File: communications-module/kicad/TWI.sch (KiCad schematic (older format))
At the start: 12 parts, among them U10 LIS3DH_breakout, U6 TPS2064, U7 I2C_connector, U8 BME280, U9 I2C_connector

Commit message: Communications Module update
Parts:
- JP17: footprint (none) -> Socket_Strips:Socket_Strip_Straight_1x02_Pitch2.54mm
- U10: footprint LIS3DH_breakout:LIS3DH_breakout -> LIS3DH_breakout:LIS3DH_breakout_vertical
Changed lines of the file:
@@
 $EndComp
 $Comp
-L GND #PWR041
+L GND #PWR50
 U 1 1 589C0F97
 P 4660 2785
-F 0 "#PWR041" H 4660 2535 50  0001 C CNN
+F 0 "#PWR50" H 4660 2535 50  0001 C CNN
 F 1 "GND" H 4660 2635 50  0000 C CNN
 F 2 "" H 4660 2785 60  0000 C CNN
@@
 $EndComp
 $Comp
-L GND #PWR042
+L GND #PWR51
 U 1 1 589C0F9D
 P 5765 2485
-F 0 "#PWR042" H 5765 2235 50  0001 C CNN
+F 0 "#PWR51" H 5765 2235 50  0001 C CNN
 F 1 "GND" H 5765 2335 50  0000 C CNN
 F 2 "" H 5765 2485 60  0000 C CNN
@@
 $EndComp
 $Comp
-L GND #PWR043
+L GND #PWR48
 U 1 1 589C0FAC
 P 4360 2270
-F 0 "#PWR043" H 4360 2020 50  0001 C CNN
+F 0 "#PWR48" H 4360 2020 50  0001 C CNN
 F 1 "GND" H 4360 2120 50  0000 C CNN
 F 2 "" H 4360 2270 60  0000 C CNN
@@
 $EndComp
 $Comp
-L GND #PWR044
+L GND #PWR49
 U 1 1 589C0FC2
 P 4525 3880
-F 0 "#PWR044" H 4525 3630 50  0001 C CNN
+F 0 "#PWR49" H 4525 3630 50  0001 C CNN
 F 1 "GND" H 4525 3730 50  0000 C CNN
 F 2 "" H 4525 3880 60  0000 C CNN
@@
 TWI_SCL
 $Comp
-L GND #PWR045
+L GND #PWR52
 U 1 1 589C0FCA
 P 5970 3885
-F 0 "#PWR045" H 5970 3635 50  0001 C CNN
+F 0 "#PWR52" H 5970 3635 50  0001 C CNN
 F 1 "GND" H 5970 3735 50  0000 C CNN
 F 2 "" H 5970 3885 60  0000 C CNN
@@
 F 0 "U10" H 7660 4860 60  0000 C CNN
 F 1 "LIS3DH_breakout" V 7535 4210 60  0000 C CNN
-F 2 "LIS3DH_breakout:LIS3DH_breakout" V 7435 4210 60  0001 C CNN
+F 2 "LIS3DH_breakout:LIS3DH_breakout_vertical" V 7435 4210 60  0001 C CNN
 F 3 "" H 7810 4710 60  0000 C CNN
 	1    7785 4285
@@
 NoConn ~ 8110 4635
 $Comp
-L GND #PWR046
+L GND #PWR58
 U 1 1 589C0FDB
 P 8580 3935
-F 0 "#PWR046" H 8580 3685 50  0001 C CNN
+F 0 "#PWR58" H 8580 3685 50  0001 C CNN
 F 1 "GND" H 8580 3785 50  0000 C CNN
 F 2 "" H 8580 3935 60  0000 C CNN
@@
 $EndComp
 $Comp
-L GND #PWR047
+L GND #PWR61
 U 1 1 589C0FF3
 P 8870 4595
-F 0 "#PWR047" H 8870 4345 50  0001 C CNN
+F 0 "#PWR61" H 8870 4345 50  0001 C CNN
 F 1 "GND" H 8870 4445 50  0000 C CNN
 F 2 "" H 8870 4595 60  0000 C CNN
@@
 $EndComp
 $Comp
-L GND #PWR048
+L GND #PWR55
 U 1 1 589C1001
 P 7795 3355
-F 0 "#PWR048" H 7795 3105 50  0001 C CNN
+F 0 "#PWR55" H 7795 3105 50  0001 C CNN
 F 1 "GND" H 7795 3205 50  0000 C CNN
 F 2 "" H 7795 3355 60  0000 C CNN
@@
 $EndComp
 $Comp
-L +3.3V #PWR049
+L +3.3V #PWR53
 U 1 1 589C100D
 P 7340 2035
-F 0 "#PWR049" H 7340 1885 50  0001 C CNN
+F 0 "#PWR53" H 7340 1885 50  0001 C CNN
 F 1 "+3.3V" H 7340 2175 50  0000 C CNN
 F 2 "" H 7340 2035 60  0000 C CNN
@@
 $EndComp
 $Comp
-L +3.3V #PWR050
+L +3.3V #PWR54
 U 1 1 589C1013
 P 7340 2365
-F 0 "#PWR050" H 7340 2215 50  0001 C CNN
+F 0 "#PWR54" H 7340 2215 50  0001 C CNN
 F 1 "+3.3V" H 7340 2505 50  0000 C CNN
 F 2 "" H 7340 2365 60  0000 C CNN
@@
 $EndComp
 $Comp
-L +3.3V #PWR051
+L +3.3V #PWR56
 U 1 1 589C102B
 P 8095 3355
-F 0 "#PWR051" H 8095 3205 50  0001 C CNN
+F 0 "#PWR56" H 8095 3205 50  0001 C CNN
 F 1 "+3.3V" H 8095 3495 50  0000 C CNN
 F 2 "" H 8095 3355 60  0000 C CNN
@@
 $EndComp
 $Comp
-L +3.3V #PWR052
+L +3.3V #PWR57
 U 1 1 589C1031
 P 8545 3790
-F 0 "#PWR052" H 8545 3640 50  0001 C CNN
+F 0 "#PWR57" H 8545 3640 50  0001 C CNN
 F 1 "+3.3V" H 8545 3930 50  0000 C CNN
 F 2 "" H 8545 3790 60  0000 C CNN
@@
 	8545 3835 8545 3790
 $Comp
-L +3.3V #PWR053
+L +3.3V #PWR59
 U 1 1 589C1039
 P 8635 4510
-F 0 "#PWR053" H 8635 4360 50  0001 C CNN
+F 0 "#PWR59" H 8635 4360 50  0001 C CNN
 F 1 "+3.3V" H 8635 4650 50  0000 C CNN
 F 2 "" H 8635 4510 60  0000 C CNN
@@
 TWI_SCL
 $Comp
-L GND #PWR054
+L GND #PWR43
 U 1 1 589C1D19
 P 2595 2690
-F 0 "#PWR054" H 2595 2440 50  0001 C CNN
+F 0 "#PWR43" H 2595 2440 50  0001 C CNN
 F 1 "GND" H 2595 2540 50  0000 C CNN
 F 2 "" H 2595 2690 60  0000 C CNN
@@
 $EndComp
 $Comp
-L +3.3V #PWR055
+L +3.3V #PWR44
 U 1 1 589C1D42
 P 2600 2930
-F 0 "#PWR055" H 2600 2780 50  0001 C CNN
+F 0 "#PWR44" H 2600 2780 50  0001 C CNN
 F 1 "+3.3V" H 2600 3070 50  0000 C CNN
 F 2 "" H 2600 2930 60  0000 C CNN
@@
 $EndComp
 $Comp
-L +3.3V #PWR056
+L +3.3V #PWR60
 U 1 1 589C1DC7
 P 8870 3875
-F 0 "#PWR056" H 8870 3725 50  0001 C CNN
+F 0 "#PWR60" H 8870 3725 50  0001 C CNN
 F 1 "+3.3V" H 8870 4015 50  0000 C CNN
 F 2 "" H 8870 3875 60  0000 C CNN
@@
 NoConn ~ 8110 4535
 $Comp
-L GND #PWR057
+L GND #PWR46
 U 1 1 58A819AA
 P 3470 5760
-F 0 "#PWR057" H 3470 5510 50  0001 C CNN
+F 0 "#PWR46" H 3470 5510 50  0001 C CNN
 F 1 "GND" H 3470 5610 50  0000 C CNN
 F 2 "" H 3470 5760 60  0000 C CNN
@@
 F 0 "JP17" H 4370 5490 50  0000 C CNN
 F 1 "Jumper_NC_Small" H 4380 5350 50  0001 C CNN
-F 2 "" H 4370 5410 60  0000 C CNN
+F 2 "Socket_Strips:Socket_Strip_Straight_1x02_Pitch2.54mm" H 4370 5410 60  0001 C CNN
 F 3 "" H 4370 5410 60  0000 C CNN
 	1    4370 5410
@@
 TWI_3V3
 $Comp
-L +3.3V #PWR058
+L +3.3V #PWR47
 U 1 1 58A81AAE
 P 4270 5410
-F 0 "#PWR058" H 4270 5260 50  0001 C CNN
+F 0 "#PWR47" H 4270 5260 50  0001 C CNN
 F 1 "+3.3V" H 4270 5550 50  0000 C CNN
 F 2 "" H 4270 5410 60  0000 C CNN
@@
 $EndComp
 $Comp
-L +3.3V #PWR059
+L +3.3V #PWR45
 U 1 1 58A8257B
 P 3235 5755
-F 0 "#PWR059" H 3235 5605 50  0001 C CNN
+F 0 "#PWR45" H 3235 5605 50  0001 C CNN
 F 1 "+3.3V" H 3235 5895 50  0000 C CNN
 F 2 "" H 3235 5755 60  0000 C CNN

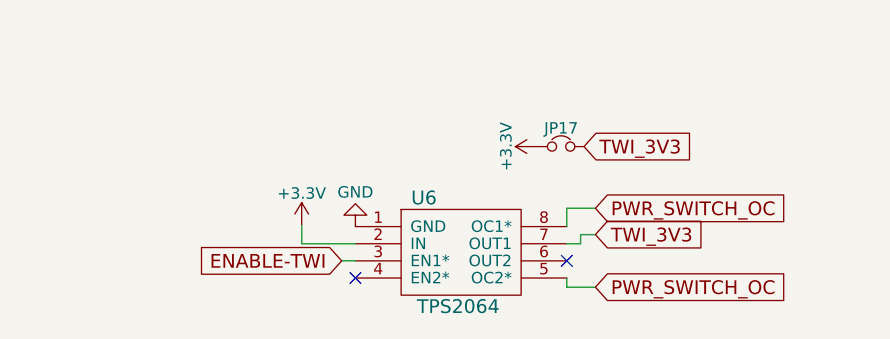
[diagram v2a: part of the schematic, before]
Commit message: Communications Module schematic update
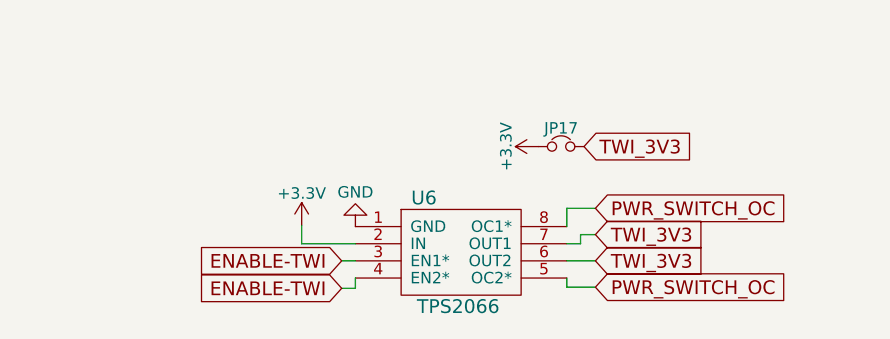
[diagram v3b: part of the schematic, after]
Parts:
- U6: value TPS2064 -> TPS2066
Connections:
- net ENABLE-TWI: now also U6.4 (EN2*)
- net TWI_3V3: now also U6.6 (OUT2)
- no-connect marks 6 -> 4
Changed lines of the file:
@@
 $EndComp
 $Comp
-L GND #PWR50
+L GND #PWR068
 U 1 1 589C0F97
 P 4660 2785
-F 0 "#PWR50" H 4660 2535 50  0001 C CNN
+F 0 "#PWR068" H 4660 2535 50  0001 C CNN
 F 1 "GND" H 4660 2635 50  0000 C CNN
 F 2 "" H 4660 2785 60  0000 C CNN
@@
 $EndComp
 $Comp
-L GND #PWR51
+L GND #PWR069
 U 1 1 589C0F9D
 P 5765 2485
-F 0 "#PWR51" H 5765 2235 50  0001 C CNN
+F 0 "#PWR069" H 5765 2235 50  0001 C CNN
 F 1 "GND" H 5765 2335 50  0000 C CNN
 F 2 "" H 5765 2485 60  0000 C CNN
@@
 $EndComp
 $Comp
-L GND #PWR48
+L GND #PWR070
 U 1 1 589C0FAC
 P 4360 2270
-F 0 "#PWR48" H 4360 2020 50  0001 C CNN
+F 0 "#PWR070" H 4360 2020 50  0001 C CNN
 F 1 "GND" H 4360 2120 50  0000 C CNN
 F 2 "" H 4360 2270 60  0000 C CNN
@@
 $EndComp
 $Comp
-L GND #PWR49
+L GND #PWR071
 U 1 1 589C0FC2
 P 4525 3880
-F 0 "#PWR49" H 4525 3630 50  0001 C CNN
+F 0 "#PWR071" H 4525 3630 50  0001 C CNN
 F 1 "GND" H 4525 3730 50  0000 C CNN
 F 2 "" H 4525 3880 60  0000 C CNN
@@
 TWI_SCL
 $Comp
-L GND #PWR52
+L GND #PWR072
 U 1 1 589C0FCA
 P 5970 3885
-F 0 "#PWR52" H 5970 3635 50  0001 C CNN
+F 0 "#PWR072" H 5970 3635 50  0001 C CNN
 F 1 "GND" H 5970 3735 50  0000 C CNN
 F 2 "" H 5970 3885 60  0000 C CNN
@@
 NoConn ~ 8110 4635
 $Comp
-L GND #PWR58
+L GND #PWR073
 U 1 1 589C0FDB
 P 8580 3935
-F 0 "#PWR58" H 8580 3685 50  0001 C CNN
+F 0 "#PWR073" H 8580 3685 50  0001 C CNN
 F 1 "GND" H 8580 3785 50  0000 C CNN
 F 2 "" H 8580 3935 60  0000 C CNN
@@
 $EndComp
 $Comp
-L GND #PWR61
+L GND #PWR074
 U 1 1 589C0FF3
 P 8870 4595
-F 0 "#PWR61" H 8870 4345 50  0001 C CNN
+F 0 "#PWR074" H 8870 4345 50  0001 C CNN
 F 1 "GND" H 8870 4445 50  0000 C CNN
 F 2 "" H 8870 4595 60  0000 C CNN
@@
 $EndComp
 $Comp
-L GND #PWR55
+L GND #PWR075
 U 1 1 589C1001
 P 7795 3355
-F 0 "#PWR55" H 7795 3105 50  0001 C CNN
+F 0 "#PWR075" H 7795 3105 50  0001 C CNN
 F 1 "GND" H 7795 3205 50  0000 C CNN
 F 2 "" H 7795 3355 60  0000 C CNN
@@
 $EndComp
 $Comp
-L +3.3V #PWR53
+L +3.3V #PWR076
 U 1 1 589C100D
 P 7340 2035
-F 0 "#PWR53" H 7340 1885 50  0001 C CNN
+F 0 "#PWR076" H 7340 1885 50  0001 C CNN
 F 1 "+3.3V" H 7340 2175 50  0000 C CNN
 F 2 "" H 7340 2035 60  0000 C CNN
@@
 $EndComp
 $Comp
-L +3.3V #PWR54
+L +3.3V #PWR077
 U 1 1 589C1013
 P 7340 2365
-F 0 "#PWR54" H 7340 2215 50  0001 C CNN
+F 0 "#PWR077" H 7340 2215 50  0001 C CNN
 F 1 "+3.3V" H 7340 2505 50  0000 C CNN
 F 2 "" H 7340 2365 60  0000 C CNN
@@
 $EndComp
 $Comp
-L +3.3V #PWR56
+L +3.3V #PWR078
 U 1 1 589C102B
 P 8095 3355
-F 0 "#PWR56" H 8095 3205 50  0001 C CNN
+F 0 "#PWR078" H 8095 3205 50  0001 C CNN
 F 1 "+3.3V" H 8095 3495 50  0000 C CNN
 F 2 "" H 8095 3355 60  0000 C CNN
@@
 $EndComp
 $Comp
-L +3.3V #PWR57
+L +3.3V #PWR079
 U 1 1 589C1031
 P 8545 3790
-F 0 "#PWR57" H 8545 3640 50  0001 C CNN
+F 0 "#PWR079" H 8545 3640 50  0001 C CNN
 F 1 "+3.3V" H 8545 3930 50  0000 C CNN
 F 2 "" H 8545 3790 60  0000 C CNN
@@
 	8545 3835 8545 3790
 $Comp
-L +3.3V #PWR59
+L +3.3V #PWR080
 U 1 1 589C1039
 P 8635 4510
-F 0 "#PWR59" H 8635 4360 50  0001 C CNN
+F 0 "#PWR080" H 8635 4360 50  0001 C CNN
 F 1 "+3.3V" H 8635 4650 50  0000 C CNN
 F 2 "" H 8635 4510 60  0000 C CNN
@@
 TWI_SCL
 $Comp
-L GND #PWR43
+L GND #PWR081
 U 1 1 589C1D19
 P 2595 2690
-F 0 "#PWR43" H 2595 2440 50  0001 C CNN
+F 0 "#PWR081" H 2595 2440 50  0001 C CNN
 F 1 "GND" H 2595 2540 50  0000 C CNN
 F 2 "" H 2595 2690 60  0000 C CNN
@@
 $EndComp
 $Comp
-L +3.3V #PWR44
+L +3.3V #PWR082
 U 1 1 589C1D42
 P 2600 2930
-F 0 "#PWR44" H 2600 2780 50  0001 C CNN
+F 0 "#PWR082" H 2600 2780 50  0001 C CNN
 F 1 "+3.3V" H 2600 3070 50  0000 C CNN
 F 2 "" H 2600 2930 60  0000 C CNN
@@
 $EndComp
 $Comp
-L +3.3V #PWR60
+L +3.3V #PWR083
 U 1 1 589C1DC7
 P 8870 3875
-F 0 "#PWR60" H 8870 3725 50  0001 C CNN
+F 0 "#PWR083" H 8870 3725 50  0001 C CNN
 F 1 "+3.3V" H 8870 4015 50  0000 C CNN
 F 2 "" H 8870 3875 60  0000 C CNN
@@
 NoConn ~ 8110 4535
 $Comp
-L GND #PWR46
+L GND #PWR084
 U 1 1 58A819AA
 P 3470 5760
-F 0 "#PWR46" H 3470 5510 50  0001 C CNN
+F 0 "#PWR084" H 3470 5510 50  0001 C CNN
 F 1 "GND" H 3470 5610 50  0000 C CNN
 F 2 "" H 3470 5760 60  0000 C CNN
@@
 P 3920 5885
 F 0 "U6" H 3770 6135 60  0000 C CNN
-F 1 "TPS2064" H 3920 5660 60  0000 C CNN
+F 1 "TPS2066" H 3920 5660 60  0000 C CNN
 F 2 "TPS2064:TPS2064" H 3920 5585 60  0001 C CNN
 F 3 "" H 3820 5660 60  0000 C CNN
@@
 TWI_3V3
 $Comp
-L +3.3V #PWR47
+L +3.3V #PWR085
 U 1 1 58A81AAE
 P 4270 5410
-F 0 "#PWR47" H 4270 5260 50  0001 C CNN
+F 0 "#PWR085" H 4270 5260 50  0001 C CNN
 F 1 "+3.3V" H 4270 5550 50  0000 C CNN
 F 2 "" H 4270 5410 60  0000 C CNN
@@
 $EndComp
 $Comp
-L +3.3V #PWR45
+L +3.3V #PWR086
 U 1 1 58A8257B
 P 3235 5755
-F 0 "#PWR45" H 3235 5605 50  0001 C CNN
+F 0 "#PWR086" H 3235 5605 50  0001 C CNN
 F 1 "+3.3V" H 3235 5895 50  0000 C CNN
 F 2 "" H 3235 5755 60  0000 C CNN
@@
 Text GLabel 4520 5795 2    60   Input ~ 0
 TWI_3V3
-NoConn ~ 4395 5910
-NoConn ~ 3470 5985
 Wire Wire Line
 	3410 5910 3470 5910
@@
 Wire Wire Line
 	8110 4335 8635 4335
+Text GLabel 3410 6030 0    60   Input ~ 0
+ENABLE-TWI
+Wire Wire Line
+	3470 5985 3470 6030
+Wire Wire Line
+	3470 6030 3410 6030
+Text GLabel 4520 5910 2    60   Input ~ 0
+TWI_3V3
+Wire Wire Line
+	4395 5910 4520 5910
 $EndSCHEMATC
